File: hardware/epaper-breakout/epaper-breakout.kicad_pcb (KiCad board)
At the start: 2 copper layers, 100 x 40.5 mm, 90 parts, among them J1 XF2M-3315-1A, J2 C10418, J3 Conn_02x06_Counter_Clockwise, J4 ED060SC4, J5 Conn_01x01_Male, J6 Conn_01x01_Male, Q1 AO3401A, Q2 AO3401A, Q3 MMBT3904, Q4 MMBT3904, Q5 AO3401A, Q6 MMBT3904, U1 MCP1700-3302E_SOT23, U10 ED060SC7, U11 TP4056, U12 CH340C, U2 LT1945, U3 LT1945, U4 XC6206PxxxMR, U5 ESP32-WROVER, U6 ED060XC5, U7 LM358, U8 74HC4094-normal, U9 MCP9700AT-ETT

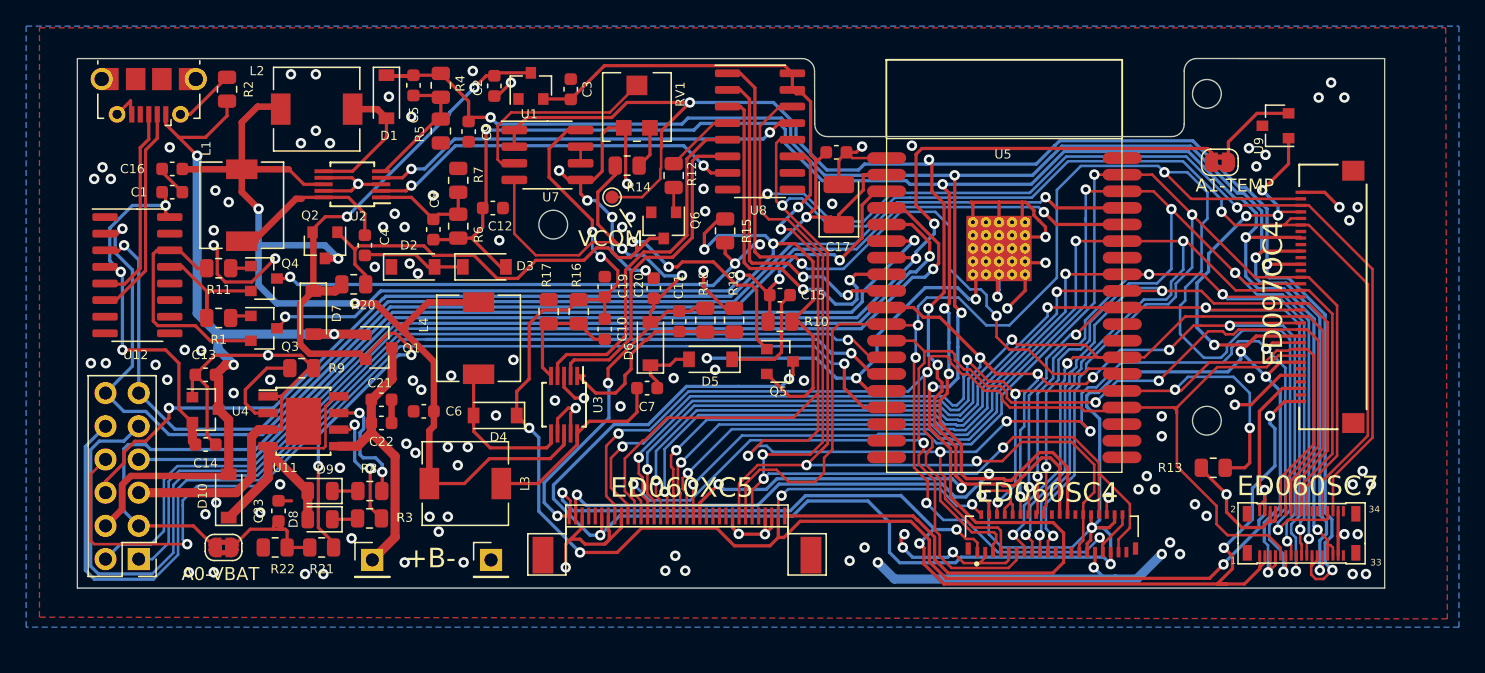
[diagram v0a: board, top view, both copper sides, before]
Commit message: Merge vroland master branch
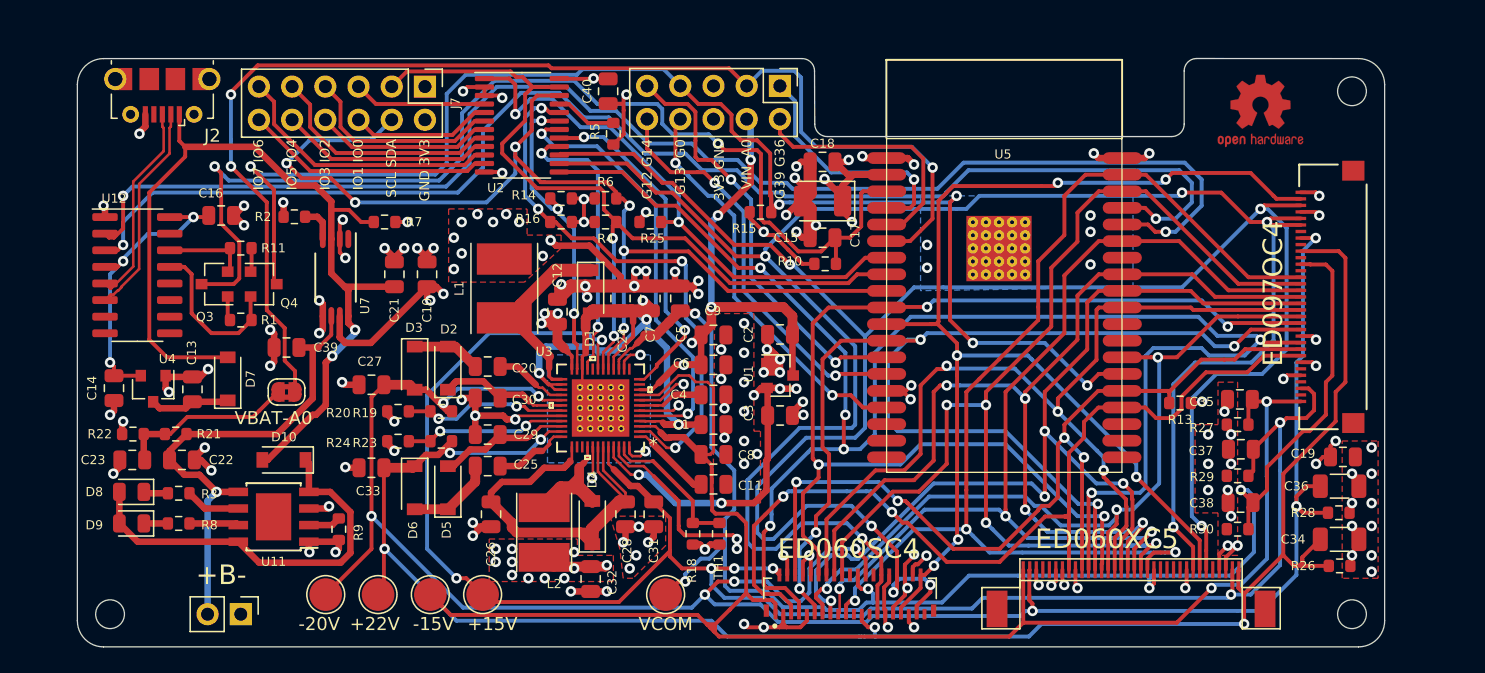
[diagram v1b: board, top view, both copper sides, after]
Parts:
- removed J6: Conn_01x01_Male, Connector_PinHeader_2.54mm:PinHeader_1x01_P2.54mm_Vertical
- removed JP_TEMP1: Jumper, Jumper:SolderJumper-2_P1.3mm_Bridged2Bar_RoundedPad1.0x1.5mm
- removed L3, L4: 22uH, Inductor_SMD:L_6.3x6.3_H3
- removed Q1, Q2, Q5: AO3401A, Package_TO_SOT_SMD:SOT-23
- removed Q6: MMBT3904, Package_TO_SOT_SMD:SOT-23
- removed R12: 1k, Resistor_SMD:R_0805_2012Metric
- removed R17: 27k, Resistor_SMD:R_0805_2012Metric
- removed RV1: 200k, epaper-breakout:EVM3ESX50B25
- removed U10: ED060SC7, epaper-breakout:AXT334124
- removed U8: 74HC4094-normal, Package_SO:SOIC-16_3.9x9.9mm_P1.27mm
- removed U9: MCP9700AT-ETT, Package_TO_SOT_SMD:SOT-23
- added C24: 4.7uF, Capacitor_SMD:C_0805_2012Metric, F.Cu at (66.5, 37.8)
- added C25: 10nF, Capacitor_SMD:C_0805_2012Metric, F.Cu at (56.4, 50.7)
- added C26: 4.7uF, Capacitor_SMD:C_0805_2012Metric, F.Cu at (56.6, 54.4)
- added C27: 2.2uF, Capacitor_SMD:C_0805_2012Metric, F.Cu at (47.5, 44.5)
- added C28: 4.7uF, Capacitor_SMD:C_0805_2012Metric, F.Cu at (66.9, 54.4)
- added C29: 100nF, Capacitor_SMD:C_0805_2012Metric, F.Cu at (56.4, 48.3)
- added C30: 100nF, Capacitor_SMD:C_0805_2012Metric, F.Cu at (56.4, 45.5)
- added C31: 4.7uF, Capacitor_SMD:C_0805_2012Metric, F.Cu at (69.1, 54.4)
- added C32: 10uF, Capacitor_SMD:C_0805_2012Metric, F.Cu at (64.3, 59.3)
- added C33: 2.2uF, Capacitor_SMD:C_0805_2012Metric, F.Cu at (47.5, 50.8)
- added C34: 1uF/50V, Capacitor_SMD:C_1206_3216Metric, F.Cu at (121.6, 56.3)
- added C35: 1uF/25V, Capacitor_SMD:C_0805_2012Metric, F.Cu at (113.9, 45.6)
- added C36: 1uF/50V, Capacitor_SMD:C_1206_3216Metric, F.Cu at (121.6, 52.2)
- added C37: 1uF/25V, Capacitor_SMD:C_0805_2012Metric, F.Cu at (114.0, 49.4)
- added C38: 1uF/25V, Capacitor_SMD:C_0805_2012Metric, F.Cu at (114.0, 53.5)
- added C39: 0.1uF, Capacitor_SMD:C_0805_2012Metric, F.Cu at (41.0, 41.6)
- added C40: 0.1uF, Capacitor_SMD:C_0805_2012Metric, F.Cu at (65.6, 22.0)
- added CC: Symbol_CreativeCommons_SilkScreenTop_Type2_Big, Symbol:Symbol_CreativeCommons_SilkScreenTop_Type2_Big, B.Cu at (117.2, 56.8)
- added J7: Conn_01x12, Connector_PinHeader_2.54mm:PinHeader_2x06_P2.54mm_Vertical, F.Cu at (51.6, 21.6)
- added R23: 1M, Resistor_SMD:R_0603_1608Metric, F.Cu at (52.8, 48.8)
- added R24: 47.5k, Resistor_SMD:R_0603_1608Metric, F.Cu at (49.5, 48.8)
- added R25: 10k, Resistor_SMD:R_0603_1608Metric, F.Cu at (68.8, 32.0)
- added R26: 47k, Resistor_SMD:R_0603_1608Metric, F.Cu at (121.6, 58.3)
- added R27: 47k, Resistor_SMD:R_0603_1608Metric, F.Cu at (113.8, 47.5)
- added R28: 47k, Resistor_SMD:R_0603_1608Metric, F.Cu at (121.5, 54.2)
- added R29: 47k, Resistor_SMD:R_0603_1608Metric, F.Cu at (113.8, 51.4)
- added R30: 100k, Resistor_SMD:R_0603_1608Metric, F.Cu at (113.8, 55.5)
- added REF**: oshw_surface, epaper-breakout:oshw_surface, F.Cu at (115.5, 23.5)
- added TH1: 10k, Resistor_SMD:R_0603_1608Metric, F.Cu at (74.1, 55.8)
- added TP2: -15V, TestPoint:TestPoint_Pad_D2.5mm, F.Cu at (52.0, 60.5)
- added TP3: -20V, TestPoint:TestPoint_Pad_D2.5mm, F.Cu at (44.0, 60.5)
- added TP4: +15V, TestPoint:TestPoint_Pad_D2.5mm, F.Cu at (56.0, 60.5)
- added TP5: VCOM, TestPoint:TestPoint_Pad_D2.5mm, F.Cu at (70.0, 60.5)
- C1, C13, C14, C15, C16, C18, C2, C22, C23, C3: footprint Capacitor_SMD:C_0603_1608Metric -> Capacitor_SMD:C_0805_2012Metric
- C10: value 4.7pF -> 22uF; footprint Capacitor_SMD:C_0603_1608Metric -> Capacitor_SMD:C_0805_2012Metric
- C11, C8: value 100pF -> 4.7uF; footprint Capacitor_SMD:C_0603_1608Metric -> Capacitor_SMD:C_0805_2012Metric
- C12, C19, C9: value 1uF -> 10uF; footprint Capacitor_SMD:C_0603_1608Metric -> Capacitor_SMD:C_0805_2012Metric
- C20: value 1uF -> 10nF; footprint Capacitor_SMD:C_0603_1608Metric -> Capacitor_SMD:C_0805_2012Metric
- C21: value 10uF -> 0.1uF; footprint Capacitor_SMD:C_0603_1608Metric -> Capacitor_SMD:C_0805_2012Metric
- C4, C7: value 0.1uF -> 4.7uF; footprint Capacitor_SMD:C_0603_1608Metric -> Capacitor_SMD:C_0805_2012Metric
- C5: value 4.7pF -> 4.7uF; footprint Capacitor_SMD:C_0603_1608Metric -> Capacitor_SMD:C_0805_2012Metric
- C6: value 4.7uF -> 22uF; footprint Capacitor_SMD:C_0603_1608Metric -> Capacitor_SMD:C_0805_2012Metric
- J3: value Conn_02x06_Counter_Clockwise -> Conn_02x05_Counter_Clockwise; footprint Connector_PinHeader_2.54mm:PinHeader_2x06_P2.54mm_Vertical -> Connector_PinHeader_2.54mm:PinHeader_2x05_P2.54mm_Vertical
- J5: value Conn_01x01_Male -> Conn_01x02_Female; footprint Connector_PinHeader_2.54mm:PinHeader_1x01_P2.54mm_Vertical -> Connector_PinHeader_2.54mm:PinHeader_1x02_P2.54mm_Vertical
- L1: value 22uH -> 4.7uH; footprint Inductor_SMD:L_6.3x6.3_H3 -> Inductor_SMD:L_Taiyo-Yuden_NR-50xx_HandSoldering
- L2: value 22uH -> 2.2uH; footprint Inductor_SMD:L_6.3x6.3_H3 -> Inductor_SMD:L_Taiyo-Yuden_NR-40xx_HandSoldering
- R1, R10, R11, R13, R15, R21, R22, R3, R8, R9: footprint Resistor_SMD:R_0805_2012Metric -> Resistor_SMD:R_0603_1608Metric
- R14: value 390k -> 10k; footprint Resistor_SMD:R_0805_2012Metric -> Resistor_SMD:R_0603_1608Metric
- R16: value 300k -> 10k; footprint Resistor_SMD:R_0805_2012Metric -> Resistor_SMD:R_0603_1608Metric
- R18: value 110k -> 43k; footprint Resistor_SMD:R_0805_2012Metric -> Resistor_SMD:R_0603_1608Metric
- R19: value 10k -> 1M; footprint Resistor_SMD:R_0805_2012Metric -> Resistor_SMD:R_0603_1608Metric
- R2: value 100k -> 400; footprint Resistor_SMD:R_0805_2012Metric -> Resistor_SMD:R_0603_1608Metric
- R20: value 10k -> 52.3k; footprint Resistor_SMD:R_0805_2012Metric -> Resistor_SMD:R_0603_1608Metric
- R4: value 2M -> 10k; footprint Resistor_SMD:R_0805_2012Metric -> Resistor_SMD:R_0603_1608Metric
- R5: value 120k -> 0; footprint Resistor_SMD:R_0805_2012Metric -> Resistor_SMD:R_0603_1608Metric
- R6: value 560k -> 10k; footprint Resistor_SMD:R_0805_2012Metric -> Resistor_SMD:R_0603_1608Metric
- R7: value 39k -> 100k; footprint Resistor_SMD:R_0805_2012Metric -> Resistor_SMD:R_0603_1608Metric
- TP1: value TestPoint_Probe -> +22V; footprint TestPoint:TestPoint_Pad_D1.0mm -> TestPoint:TestPoint_Pad_D2.5mm
- U2: value LT1945 -> PCA9535PW; footprint Package_SO:MSOP-10_3x3mm_P0.5mm -> Package_SO:TSSOP-24_4.4x7.8mm_P0.65mm
- U3: value LT1945 -> TPS651851RSLR; footprint Package_SO:MSOP-10_3x3mm_P0.5mm -> tps65185:TPS651851RSLR
- U7: value LM358 -> TPS2113APW; footprint Package_SO:SOP-8_3.76x4.96mm_P1.27mm -> epaper-breakout:TPS2113APW
- moved J3 61.0 mm to (78.7, 21.6), turned to 270 degrees
- moved C19 57.9 mm to (121.8, 50.0), turned to 0 degrees
- moved C1 45.8 mm to (73.7, 47.5), turned to 0 degrees
- moved H2 45.1 mm to (27.5, 62.0)
- moved L2 36.8 mm to (60.7, 55.8), turned to 90 degrees
- moved TP1 35.3 mm to (48.0, 60.5)
- moved U6 35.0 mm to (105.6, 58.6)
- moved C3 29.7 mm to (78.8, 46.8), turned to 180 degrees
- moved U1 29.2 mm to (78.8, 43.7), turned to 0 degrees
- moved C4 29.0 mm to (73.7, 45.2), turned to 180 degrees
- moved C2 29.0 mm to (78.8, 40.6), turned to 0 degrees
- moved C8 27.5 mm to (73.7, 49.8), turned to 180 degrees
- moved C5 26.1 mm to (71.1, 37.8), turned to 270 degrees
- moved C9 24.4 mm to (73.7, 40.6), turned to 0 degrees
- moved R19 23.5 mm to (52.8, 46.5), turned to 180 degrees
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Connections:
- net Net-(J2-Pad2) renamed /USB_D-
- net Net-(J2-Pad3) renamed /USB_D+
- C1 pad 1: SW_VIN -> /VNEG_IN
- C10 pad 1: Net-(C10-Pad1) -> GND
- C10 pad 2: /15V -> SW_VIN
- C11 pad 1: Net-(C11-Pad1) -> GND
- C11 pad 2: /-15V -> Net-(C11-Pad2)
- C12 pad 1: GND -> SW_VIN
- C12 pad 2: /-20V -> GND
- C13 pad 1: VBUS -> Net-(C13-Pad1)
- C19 pad 1: GND -> EPD_VDD
- C19 pad 2: /15V -> GND
- C2 pad 2: VIN -> SW_VIN
- C20 pad 1: GND -> Net-(C20-Pad1)
- C20 pad 2: /-15V -> Net-(C20-Pad2)
- C21 pad 1: BAT+ -> VBUS
- C4 pad 1: Net-(C4-Pad1) -> GND
- C5 pad 1: Net-(C5-Pad1) -> GND
- C5 pad 2: /+22V -> /EP_VCOM
- C6 pad 1: SW_VIN -> GND
- C6 pad 2: GND -> SW_VIN
- C7 pad 1: Net-(C7-Pad1) -> /VNEG_IN
- C7 pad 2: Net-(C7-Pad2) -> GND
- C8 pad 1: Net-(C8-Pad1) -> GND
- C8 pad 2: /-20V -> /-15V
- C9 pad 1: GND -> SW_VIN
- C9 pad 2: /+22V -> GND
- D1 pad 1: /+22V -> Net-(D1-Pad1)
- D1 pad 2: Net-(D1-Pad2) -> /VNEG_IN
- D2 pad 1: GND -> Net-(C30-Pad1)
- D2 pad 2: Net-(C4-Pad1) -> Net-(C20-Pad1)
- D3 pad 1: Net-(C4-Pad1) -> Net-(C20-Pad1)
- D4 pad 1: /15V -> Net-(C26-Pad2)
- D5 pad 1: GND -> Net-(C25-Pad1)
- D5 pad 2: Net-(C7-Pad1) -> Net-(C29-Pad2)
- D6 pad 1: Net-(C7-Pad1) -> /+22V
- D6 pad 2: /-15V -> Net-(C25-Pad1)
- D7 pad 1: VIN -> Net-(C13-Pad1)
- J1 pad 2: (no net) -> Net-(J1-Pad2)
- J1 pad 21: (no net) -> Net-(J1-Pad21)
- J1 pad 23: (no net) -> Net-(J1-Pad23)
- J1 pad 25: (no net) -> Net-(J1-Pad25)
- J1 pad 27: (no net) -> Net-(J1-Pad27)
- J1 pad 34: (no net) -> Net-(J1-Pad34)
- J1 pad 35: (no net) -> Net-(J1-Pad35)
- J1 pad 4: (no net) -> Net-(J1-Pad4)
- J1 pad 6: (no net) -> Net-(J1-Pad6)
- J2 pad 4: (no net) -> Net-(J2-Pad4)
- J3 pad 4: VBUS -> SW_VIN
- J3 pad 7: /A1 -> /IO0
- J4 pad 20: (no net) -> Net-(J4-Pad20)
- J4 pad 21: (no net) -> Net-(J4-Pad21)
- J4 pad 25: (no net) -> Net-(J4-Pad25)
- J4 pad 26: (no net) -> Net-(J4-Pad26)
- J4 pad 39: (no net) -> Net-(J4-Pad39)
- J5 pad 1: BAT+ -> GND
- L1 pad 1: Net-(C4-Pad2) -> Net-(D1-Pad1)
- L1 pad 2: SW_VIN -> GND
- L2 pad 1: Net-(D1-Pad2) -> SW_VIN
- L2 pad 2: SW_VIN -> Net-(D4-Pad2)
- R14 pad 1: /-15V -> /+3.3V
- R14 pad 2: Net-(R14-Pad2) -> /TPS_PWR_GOOD
- R16 pad 1: /15V -> /+3.3V
- R16 pad 2: Net-(C10-Pad1) -> /TPS_nINT
- R18 pad 1: /-15V -> GND
- R18 pad 2: Net-(C11-Pad1) -> Net-(R18-Pad2)
- R19 pad 1: Net-(C11-Pad1) -> /-20V
- R19 pad 2: GND -> Net-(R19-Pad2)
- R2 pad 1: GND -> Net-(R2-Pad1)
- R2 pad 2: VBUS -> GND
- R20 pad 1: Net-(Q2-Pad1) -> Net-(R19-Pad2)
- R20 pad 2: VIN -> GND
- R21 pad 1: VIN -> BAT+
- R4 pad 1: /+22V -> /+3.3V
- R4 pad 2: Net-(C5-Pad1) -> /SDA
- R5 pad 1: Net-(C5-Pad1) -> Net-(R5-Pad1)
- R6 pad 1: /-20V -> /+3.3V
- R6 pad 2: Net-(C8-Pad1) -> /SCL
- R7 pad 1: Net-(C8-Pad1) -> VBUS
- TP1 pad 1: /EP_VCOM -> /+22V
- U1 pad 3: VIN -> SW_VIN
- U11 pad 9: (no net) -> Net-(U11-Pad9)
- U12 pad 10: (no net) -> Net-(U12-Pad10)
- U12 pad 11: (no net) -> Net-(U12-Pad11)
- U12 pad 12: (no net) -> Net-(U12-Pad12)
- U12 pad 15: (no net) -> Net-(U12-Pad15)
- U12 pad 7: (no net) -> Net-(U12-Pad7)
- U12 pad 8: (no net) -> Net-(U12-Pad8)
- U12 pad 9: (no net) -> Net-(U12-Pad9)
- U2 pad 1: Net-(C8-Pad1) -> /~GPIO_INTR
- U2 pad 10: Net-(C4-Pad2) -> Net-(J7-Pad11)
- U2 pad 2: /CTRL-20V -> GND
- U2 pad 4: /CTRL+22V -> Net-(J7-Pad5)
- U2 pad 5: Net-(C5-Pad1) -> Net-(J7-Pad6)
- U2 pad 6: Net-(D1-Pad2) -> Net-(J7-Pad7)
- U2 pad 7: GND -> Net-(J7-Pad8)
- U2 pad 8: SW_VIN -> Net-(J7-Pad9)
- U2 pad 9: GND -> Net-(J7-Pad10)
- U3 pad 1: Net-(C11-Pad1) -> Net-(C11-Pad2)
- U3 pad 10: Net-(C7-Pad2) -> SW_VIN
- U3 pad 2: /CTRL-15V -> /TPS_nINT
- U3 pad 3: GND -> /-15V
- U3 pad 4: /CTRL+15V -> /VNEG_IN
- U3 pad 5: Net-(C10-Pad1) -> /TPS_WAKEUP
- U3 pad 6: Net-(D4-Pad2) -> GND
- U3 pad 7: GND -> Net-(C4-Pad2)
- U3 pad 8: SW_VIN -> GND
- U3 pad 9: GND -> /-15V
- U4 pad 3: VBUS -> Net-(C13-Pad1)
- U5 pad 17: (no net) -> Net-(U5-Pad17)
- U5 pad 18: (no net) -> Net-(U5-Pad18)
- U5 pad 19: (no net) -> Net-(U5-Pad19)
- U5 pad 20: (no net) -> Net-(U5-Pad20)
- U5 pad 21: (no net) -> Net-(U5-Pad21)
- U5 pad 22: (no net) -> Net-(U5-Pad22)
- U5 pad 27: (no net) -> Net-(U5-Pad27)
- U5 pad 28: (no net) -> Net-(U5-Pad28)
- U5 pad 32: (no net) -> Net-(U5-Pad32)
- U5 pad 7: /A1 -> /~GPIO_INTR
- U5 pad 8: Net-(U5-Pad8) -> /SDA
- U5 pad 9: Net-(U5-Pad9) -> /SCL
- U6 pad 22: (no net) -> Net-(U6-Pad22)
- U6 pad 23: (no net) -> Net-(U6-Pad23)
- U6 pad 24: (no net) -> Net-(U6-Pad24)
- U6 pad 25: (no net) -> Net-(U6-Pad25)
- U6 pad 30: (no net) -> Net-(U6-Pad30)
- U6 pad 4: (no net) -> Net-(U6-Pad4)
- U6 pad 5: (no net) -> Net-(U6-Pad5)
- U7 pad 1: /EP_VCOM -> Net-(U7-Pad1)
- U7 pad 2: /EP_VCOM -> GND
- U7 pad 3: Net-(RV1-Pad2) -> VBUS
- U7 pad 4: /-15V -> Net-(R2-Pad1)
- U7 pad 6: Net-(U7-Pad6) -> BAT+
- U7 pad 7: Net-(U7-Pad6) -> SW_VIN
- U7 pad 8: /15V -> VBUS
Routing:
- net EPD_VDD: track 184.5 -> 38.9 mm, vias 12 -> 13
- net /A1: track 100.9 -> 0.00 mm, vias 2 -> 0
- net /SCL: track 0.00 -> 83.4 mm, vias 0 -> 6
- net /SDA: track 0.00 -> 66.3 mm, vias 0 -> 2
- net /VNEG_IN: track 0.00 -> 63.3 mm, vias 0 -> 4
- net VIN: track 63.1 -> 0.00 mm, vias 4 -> 0
- net /SENSOR_VP: track 79.9 -> 18.9 mm
- net /SENSOR_VN: track 80.0 -> 19.8 mm, vias 1 -> 0
- net /EP_VCOM: track 177.6 -> 119.2 mm, vias 8 -> 5
- net /EP_CKV: track 149.6 -> 95.3 mm
- net /MISO: track 84.9 -> 31.4 mm, vias 1 -> 2
- net /SCLK: track 85.8 -> 32.8 mm, vias 1 -> 2
- net Net-(Q2-Pad1): track 51.1 -> 0.00 mm, vias 2 -> 0
- net /+3.3V: track 135.8 -> 85.8 mm, vias 4 -> 13
- net /MOSI: track 79.4 -> 31.1 mm
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- added copper zone on In2.Cu, net /+3.3V
- added copper zone on B.Cu, net /VNEG_IN
- added copper zone on In2.Cu, net EPD_VDD
- added copper zone on In1.Cu, net GND
- added copper zone on F.Cu, net SW_VIN
- added copper zone on In2.Cu, net SW_VIN
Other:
- board size 100 x 40.5 mm -> 100 x 45 mm
- copper layers 2 -> 4
- board text added: "3V3 GND"
- board text added: "G12 G14"
- board text added: "G13 G0"
- board text added: "G39 G36"
- board text added: "GND 3V3"
- board text added: "IO1 IO0"
- board text added: "IO3 IO2"
- board text added: "IO5 IO4"
- board text added: "IO7 IO6"
- board text added: "SCL SDA"
- board text added: "VBAT-A0"
- board text added: "VIN A0"
- board text added: "epdiy v6 by Valentin Roland 2021 Thanks to the epdiy contributors! For sources and documentation visit https://github.com/vroland/epdiy"
- board text removed: "A0-VBAT"
- board text removed: "A1-TEMP"
- board text removed: "ED060SC7"
- board text removed: "RX TX 14 12 35/Tmp 13 GND 3.3V 34 5V 36 39"
- board text removed: "VCOM"
- board text removed: "epdiy v5 by Valentin Roland 2021 Thanks to the epdiy contributors!"
